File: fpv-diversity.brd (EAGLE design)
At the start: 38.1 x 70.8 mm, 32 parts, among them U1 LM1881M/NOPB, U2 LM1881M/NOPB, U3 LM1881M/NOPB, U4 MAX4545CAP+

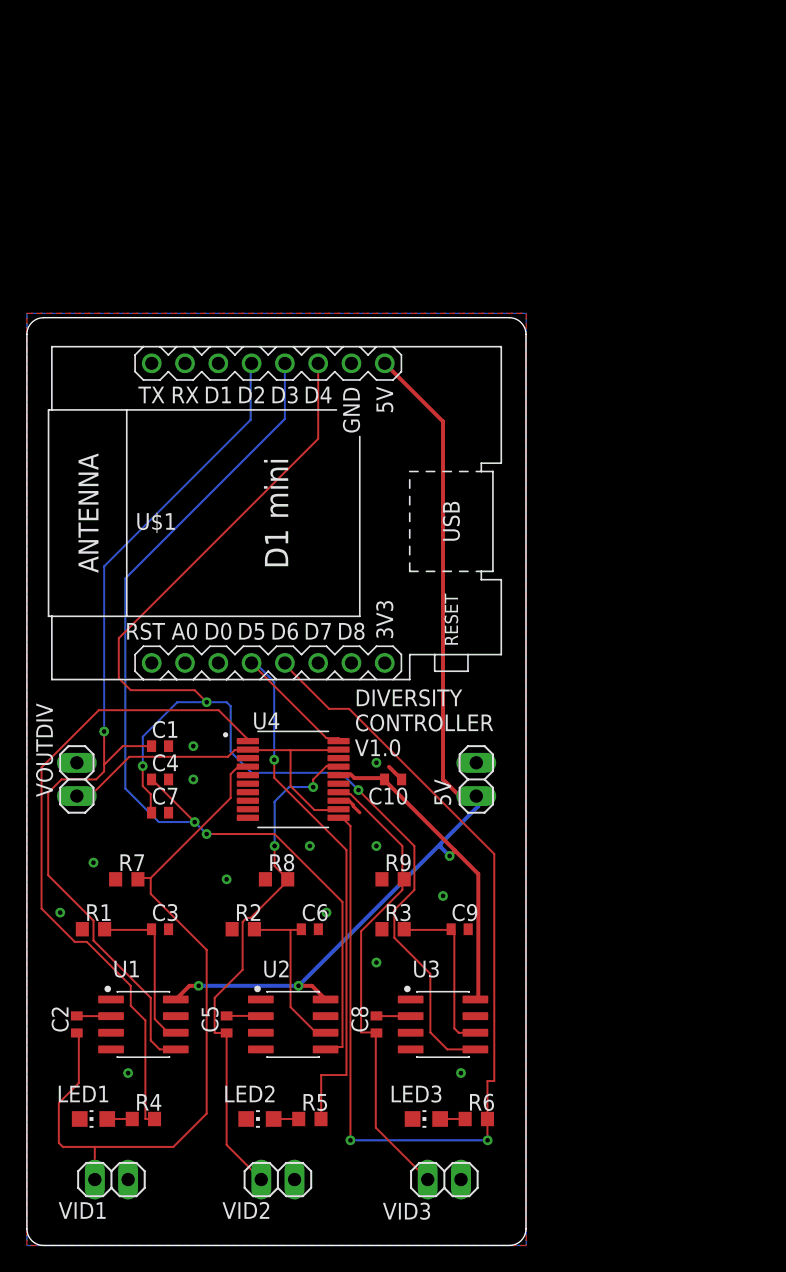
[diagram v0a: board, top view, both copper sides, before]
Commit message: PCB updates
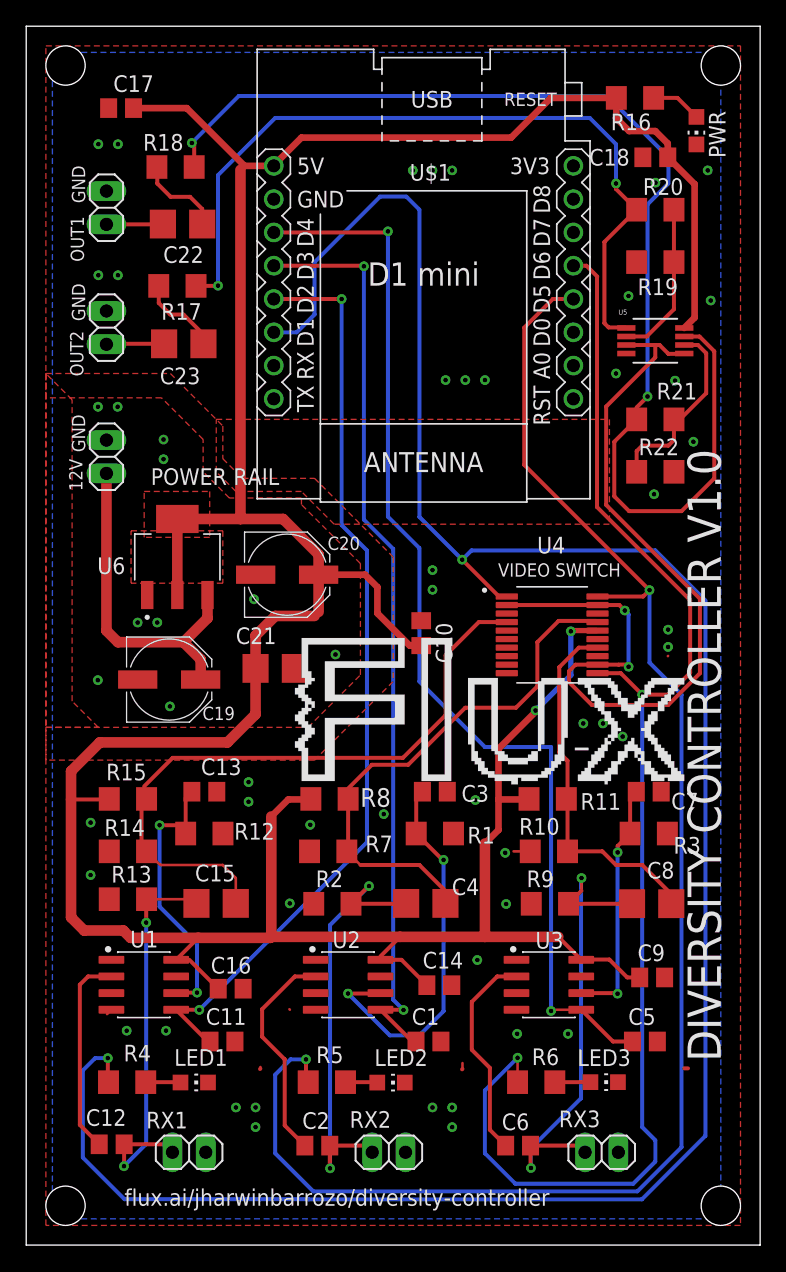
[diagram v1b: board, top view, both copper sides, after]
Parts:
- removed 5V, VID1, VID2, VID3, VOUTDIV: (no value), pinhead:1X02
- added 12V, OUT1, OUT2, RX1, RX2, RX3: (no value), pinhead:1X02
- added C11: 1nF, rcl:C0805
- added C12, C13, C14, C16, C17, C18: 100nF, rcl:C0805
- added C15: 47uF, rcl:CT3528
- added C19: 10uF, rcl:PANASONIC_D
- added C20: 33uF, rcl:PANASONIC_D
- added C21: 4.7uF, rcl:CT3528
- added C22, C23: 470uF, rcl:CT3528
- added PWR: (no value), led:CHIP-LED0805
- added R10, R14: 1K, rcl:R1206
- added R11, R15: 4.7K, rcl:R1206
- added R12: 680K, rcl:R1206
- added R13, R17, R18: 75, rcl:R1206
- added R16: 470, rcl:R1206
- added R19, R20, R21, R22: 499, rcl:R1206
- added U5: LT6206CMS8PBF, LT6206CMS8PBF:MSOP-8_MS
- added U6: LM1117IMP-5.0-NOPB, LM1117IMP-5.0-NOPB:SOT230P700X180-4N
- C1, C10, C2, C3, C6, C9: device rcl:C0402 -> rcl:C0805
- C4: value 1nF -> 47uF; device rcl:C0402 -> rcl:CT3528
- C5: value 100nF -> 1nF; device rcl:C0402 -> rcl:C0805
- C7: value 1nF -> 100nF; device rcl:C0402 -> rcl:C0805
- C8: value 100nF -> 47uF; device rcl:C0402 -> rcl:CT3528
- R1, R3, R4, R5, R6, R9: device rcl:R0603 -> rcl:R1206
- R2: value 680K -> 75; device rcl:R0603 -> rcl:R1206
- R7: value 75 -> 1K; device rcl:R0603 -> rcl:R1206
- R8: value 75 -> 4.7K; device rcl:R0603 -> rcl:R1206
- moved C7 37.3 mm to (47.4, 34.6)
- moved C5 31.9 mm to (47.2, 15.6), turned to 0 degrees
- moved C1 30.5 mm to (30.6, 15.6)
- moved R1 27.1 mm to (31.1, 31.4), turned to 180 degrees
- moved C3 23.4 mm to (31.1, 34.6)
- moved C8 22.9 mm to (47.7, 26.1), turned to 180 degrees
- moved C6 22.9 mm to (37.5, 7.62), turned to 180 degrees
- moved U4 22.6 mm to (40.1, 46.6)
- moved C4 22.4 mm to (30.4, 26.1), turned to 180 degrees
- moved U$1 21.4 mm to (30.3, 74.1), turned to 180 degrees
- moved R3 20.8 mm to (47.4, 31.4), turned to 180 degrees
- moved C2 20.5 mm to (22.2, 7.62), turned to 180 degrees
- moved R7 15.5 mm to (23.0, 30.1)
- moved C9 15.1 mm to (47.7, 20.5)
- moved LED3 13.9 mm to (44.0, 12.5), turned to 270 degrees
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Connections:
- removed net 1N1: U$1.JP2.3
- removed net N$6: C8.2, U3.2
- removed net VOUT: U4.12, U4.19, U4.2, VOUTDIV.1
- new net 5V: C10.1, C14.1, C16.1, C17.1, C18.1, C20.+, C21.+, C9.1, R11.2, R15.2, R16.2, R8.2, U$1.JP2.8, U1.8, U2.8, U3.8, U4.16, U5.8, U6.2, U6.4
- new net N$10: C13.1, R12.2, U1.6
- new net N$11: C12.2, U1.2
- new net N$12: R19.1, R20.2, U5.2
- new net N$13: R18.2, R21.1, U5.7
- new net N$14: R21.2, R22.1, U5.6
- new net N$15: R17.1, R20.1, U5.1
- new net N$16: C22.+, R18.1
- new net N$17: C23.+, R17.2
- new net PRE-VOUT: U4.12, U4.19, U4.2, U5.3, U5.5
- new net VID1: C12.1, C15.-, R13.2, RX1.1
- new net VID2: C2.1, C4.-, R2.2, RX2.1
- new net VID3: C6.1, C8.-, R9.2, RX3.1
- new net VOUT1: C22.-, OUT1.1
- new net VOUT2: C23.-, OUT2.1
- net BPOUT1: now also C11.1; no longer C1.1
- net BPOUT2: now also C1.1; no longer C4.1
- net BPOUT3: now also C5.1; no longer C7.1
- net GND: now also 12V.2, C11.2, C13.2, C14.2, C16.2, C17.2, C18.2, C19.-, C20.-, C21.-, C5.2, OUT1.2, OUT2.2, PWR.C, R10.1, R12.1, R13.1, R14.1, R19.2, R22.2, RX1.2, RX2.2, RX3.2, U5.4, U6.1; no longer 5V.2, C4.2, C6.2, R8.1, VID1.2, VID2.2, VID3.2, VOUTDIV.2
- net IN1: now also U$1.JP2.3
- net N$1: now also C7.1, R3.2, U3.6; no longer C2.2, U1.2
- net N$2: now also C3.1, R1.2; no longer C6.1, R2.2
- net N$3: now also C2.2, U2.2; no longer C3.1, R1.2, U1.6
- net N$4: now also PWR.A, R16.1; no longer C5.2, U2.2
- net N$5: now also C6.2, U3.2; no longer C9.1, R3.2, U3.6
- net N01: now also C15.+, R14.2, R15.1; no longer C2.1, R7.2, VID1.1
- net N02: now also C4.+, R7.2, R8.1; no longer C5.1, R8.2, VID2.1
- net N03: now also C8.+, R10.2, R11.1; no longer C8.1, R9.2, VID3.1
- net VCC: now also 12V.1, C19.+, U6.3; no longer 5V.1, C10.1, U$1.JP2.8, U1.8, U2.8, U3.8, U4.16
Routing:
- net 5V: track 0.00 -> 266.1 mm, vias 0 -> 2
- net IN1: track 49.9 -> 173.7 mm, vias 0 -> 2
- net N$13: track 0.00 -> 90.9 mm, vias 0 -> 2
- net IN2: track 49.2 -> 120.6 mm, vias 1 -> 2
- net VCC: track 94.9 -> 26.0 mm, vias 3 -> 0
- net PRE-VOUT: track 0.00 -> 65.2 mm, vias 0 -> 2
- net N$15: track 0.00 -> 60.3 mm, vias 0 -> 2
- net VID3: track 0.00 -> 37.0 mm, vias 0 -> 2
- net VID2: track 0.00 -> 34.1 mm, vias 0 -> 2
- net VID1: track 0.00 -> 30.6 mm, vias 0 -> 2
- net VOUT: track 28.7 -> 0.00 mm
- net IN3: track 80.0 -> 104.7 mm
- net N$10: track 0.00 -> 21.2 mm, vias 0 -> 2
- net N$2: track 13.0 -> 29.7 mm, vias 0 -> 2
- net N$1: track 2.62 -> 18.8 mm, vias 0 -> 2
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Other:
- board size 38.1 x 70.8 mm -> 56 x 93 mm
- board text added: "GND"
- board text added: "POWER RAIL"
- board text added: "VIDEO SWITCH"
- board text added: "flux.ai/jharwinbarrozo/diversity-controller"
- board text removed: "Made in Flux.ai"
- board text removed: "jharwinbarrozo"

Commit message: .brd cleanup
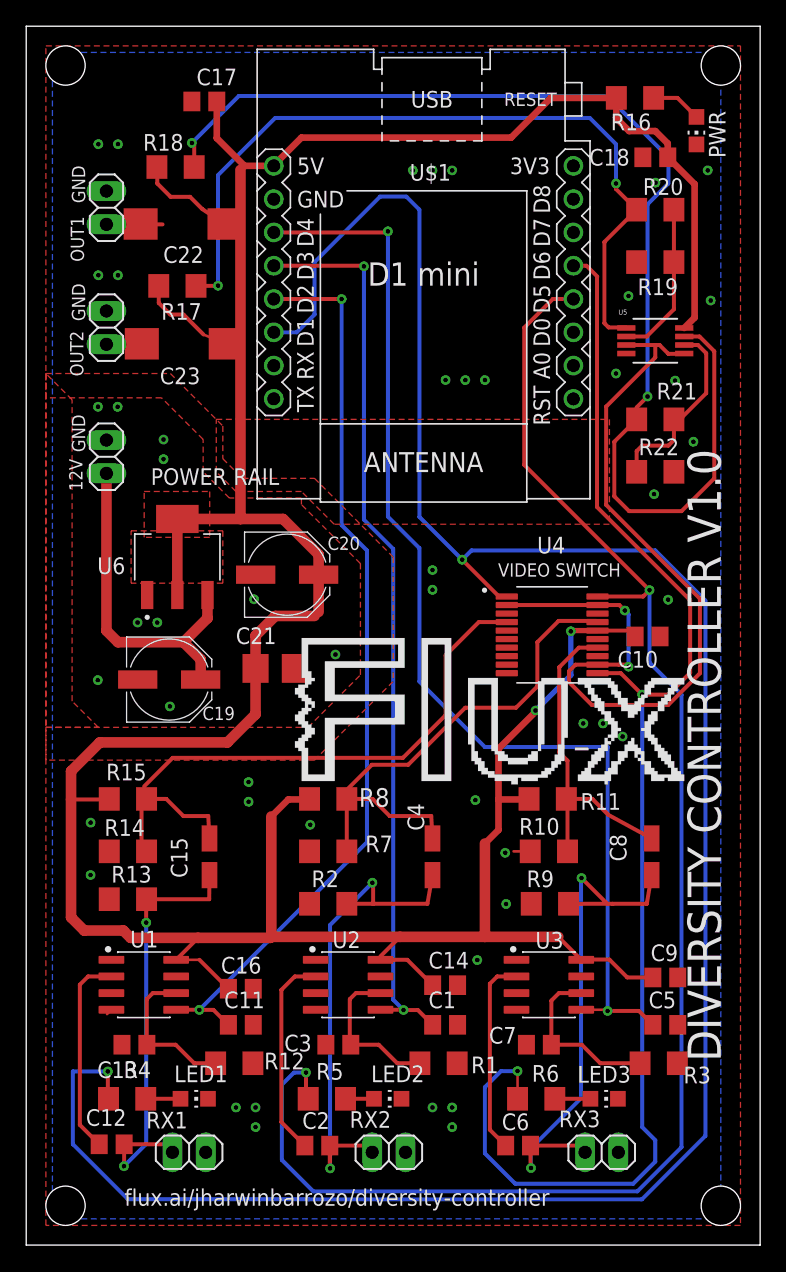
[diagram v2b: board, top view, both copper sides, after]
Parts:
- C15, C4, C8: device rcl:CT3528 -> rcl:CT3216
- C22, C23: device rcl:CT3528 -> rcl:CT7343
- moved C7 21.0 mm to (39.1, 15.3), turned to 180 degrees
- moved C3 20.7 mm to (23.8, 15.3), turned to 180 degrees
- moved C13 20.0 mm to (8.20, 15.3), turned to 180 degrees
- moved R12 17.7 mm to (15.8, 13.9)
- moved R3 17.5 mm to (48.2, 13.9)
- moved R1 17.5 mm to (31.4, 13.9)
- moved C10 17.3 mm to (47.4, 46.5), turned to 0 degrees
- moved C17 6.37 mm to (13.5, 87.3)
- moved C15 3.59 mm to (13.9, 29.7), turned to 270 degrees
- moved C4 3.59 mm to (30.9, 29.7), turned to 270 degrees
- moved C8 3.58 mm to (47.7, 29.7), turned to 270 degrees
- moved C5 2.01 mm to (48.7, 16.8)
- moved C11 1.89 mm to (16.3, 16.8)
- moved C1 1.80 mm to (31.9, 16.8)
- moved LED3 1.27 mm to (44.0, 11.2)
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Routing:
- net N$2: track 29.7 -> 11.9 mm, vias 2 -> 0
- net 5V: track 266.1 -> 255.5 mm
- net N$10: track 21.2 -> 11.7 mm, vias 2 -> 0
- net N$1: track 18.8 -> 13.2 mm, vias 2 -> 0
- net VID2: track 34.1 -> 38.3 mm
- net VID3: track 37.0 -> 40.8 mm
- net N01: track 50.6 -> 47.5 mm
- net BPOUT3: track 83.6 -> 86.6 mm
- net VID1: track 30.6 -> 33.3 mm
- net N03: track 28.0 -> 25.4 mm
- net GND: track 6.45 -> 4.41 mm, vias 56 -> 49
- net N02: track 40.9 -> 39.2 mm
- net VOUT2: track 4.42 -> 2.72 mm
- net VOUT1: track 4.32 -> 5.96 mm
- net IN2: track 120.6 -> 119.2 mm
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
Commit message: Updates
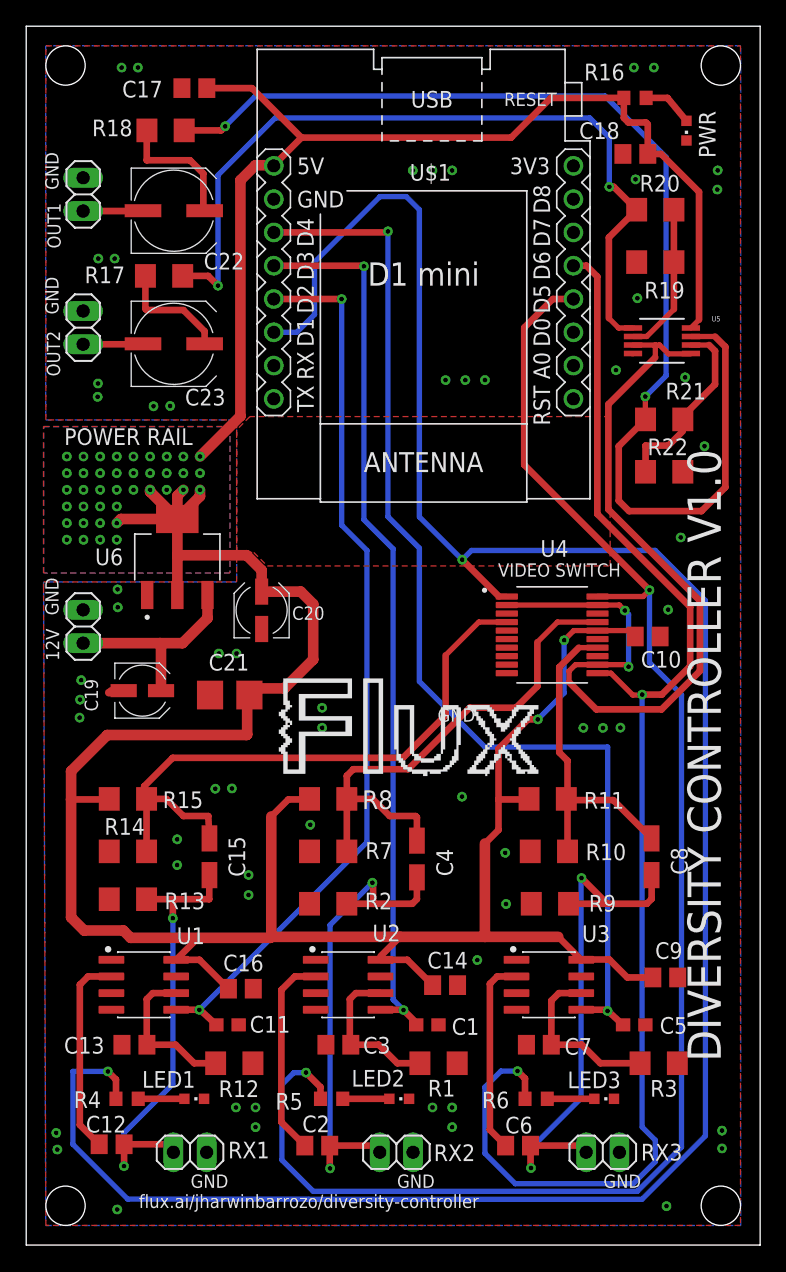
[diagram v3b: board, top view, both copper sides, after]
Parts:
- C1, C11, C5: device rcl:C0805 -> rcl:C0603
- C19, C20: device rcl:PANASONIC_D -> rcl:UD-4X5,8_NICHICON
- C22, C23: device rcl:CT7343 -> rcl:UD-6,3X7,7_NICHICON
- LED1, LED2, LED3, PWR: device led:CHIP-LED0805 -> led:CHIPLED_0603
- R16, R4, R5, R6: value 470 -> 120; device rcl:R1206 -> rcl:R0603
- moved 12V 13.1 mm to (4.29, 47.2)
- moved C21 4.02 mm to (15.5, 42.0), turned to 180 degrees
- moved C20 3.34 mm to (17.9, 48.5), turned to 90 degrees
- moved R18 2.90 mm to (10.6, 85.1)
- moved C5 2.37 mm to (46.3, 16.8)
- moved C19 2.22 mm to (8.81, 42.3)
- moved OUT1 2.05 mm to (4.29, 80.2)
- moved OUT2 1.78 mm to (4.29, 70.0)
- moved C18 1.55 mm to (46.4, 83.3)
- moved C1 1.35 mm to (30.6, 16.8)
- moved C17 1.27 mm to (12.8, 88.3)
- moved R17 1.27 mm to (10.5, 74.0)
- moved C22 1.22 mm to (11.2, 79.0), turned to 0 degrees
- moved C4 1.20 mm to (29.8, 29.5)
- moved C11 1.02 mm to (15.3, 16.8)
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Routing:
- net 5V: track 255.5 -> 267.2 mm, vias 2 -> 41
- net VCC: track 26.0 -> 15.7 mm
- net N$16: track 7.55 -> 9.89 mm
- net BPOUT3: track 86.6 -> 84.3 mm
- net VOUT2: track 2.72 -> 4.58 mm
- net N$8: track 2.17 -> 3.56 mm
- net N$15: track 60.3 -> 61.7 mm
- net VOUT1: track 5.96 -> 4.58 mm
- net N$17: track 7.55 -> 8.69 mm
- net BPOUT2: track 69.4 -> 68.3 mm
- net BPOUT1: track 70.0 -> 69.0 mm
- net VID1: track 33.3 -> 34.2 mm
- net N$7: track 2.65 -> 3.52 mm
- net N$9: track 2.72 -> 3.59 mm
- net N01: track 47.5 -> 48.2 mm
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- added copper zone on layer 1, net 5V
- added copper zone on layer 16, net 5V
